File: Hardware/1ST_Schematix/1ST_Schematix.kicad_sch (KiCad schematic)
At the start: 6 parts, among them SW101 SW_Push

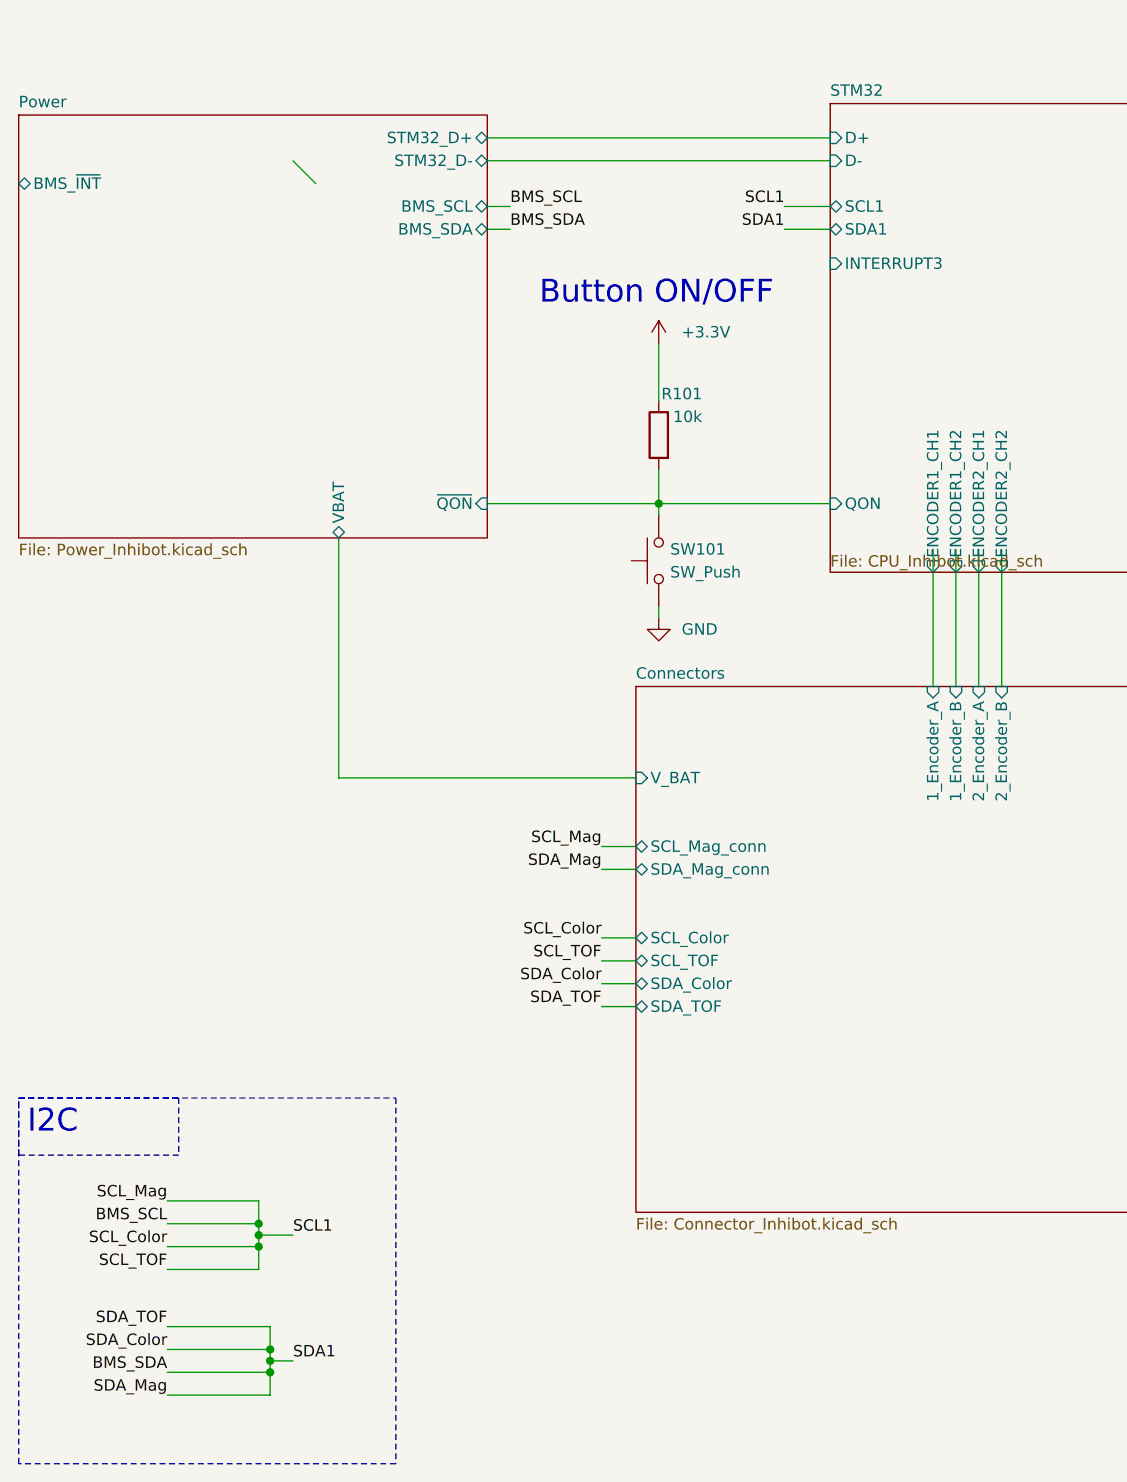
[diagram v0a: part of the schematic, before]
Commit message: Update
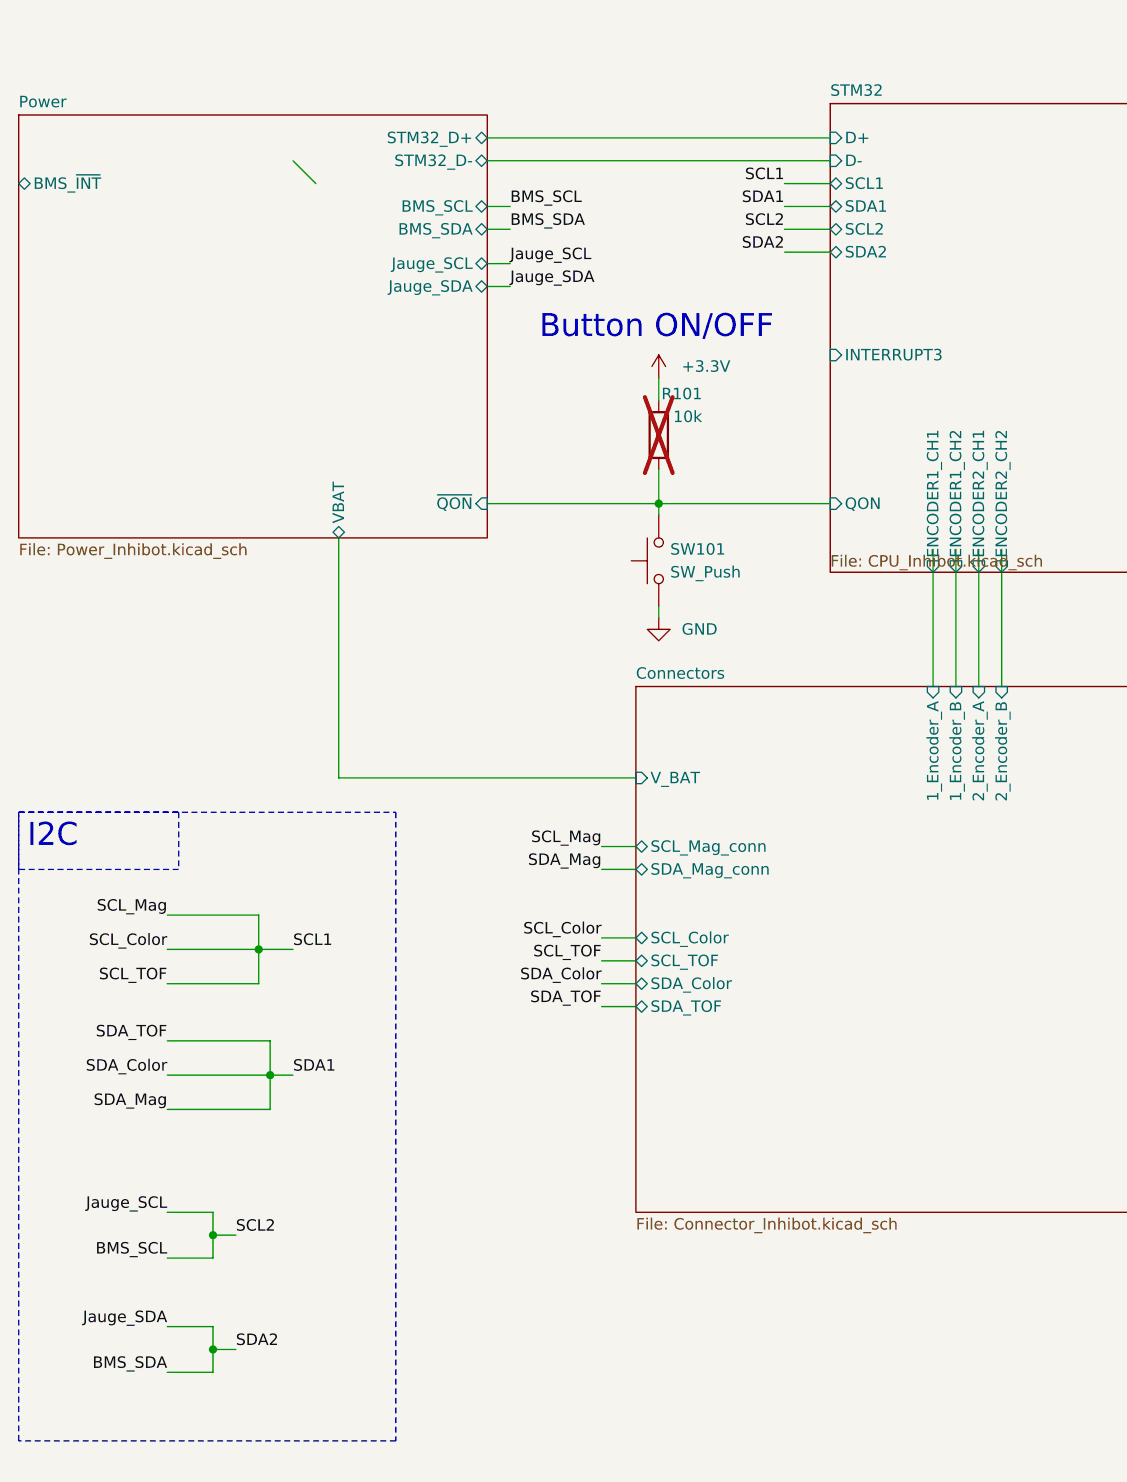
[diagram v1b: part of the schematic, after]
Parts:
- R101: now not fitted
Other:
- sheet Power ports: added Jauge_SCL, Jauge_SDA; removed none
- sheet STM32 ports: added SCL2, SDA2; removed none
